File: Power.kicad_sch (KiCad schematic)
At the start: 38 parts, among them IC1 LM66200DRLR, J22 Conn_01x02, U10 LP2985-3.3, U9 AP63203WU

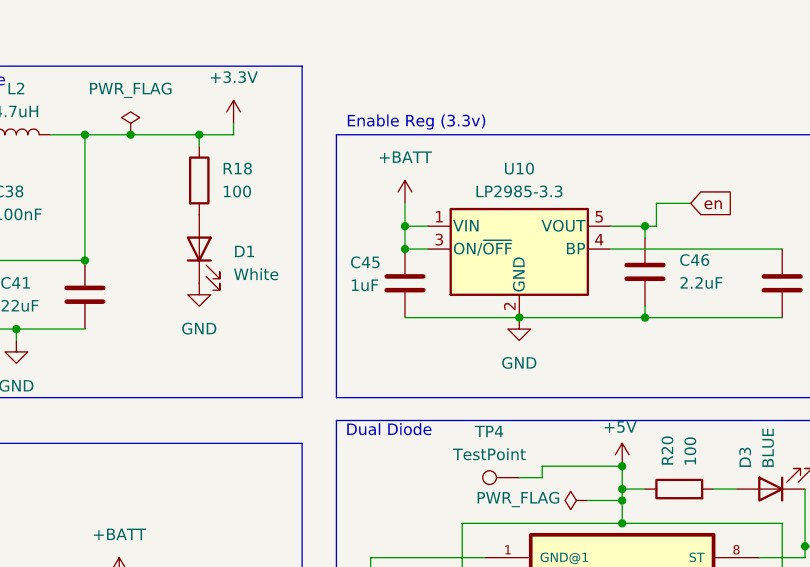
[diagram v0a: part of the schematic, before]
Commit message: v1.0 DONE6️⃣7️⃣🚀⚡️🔋
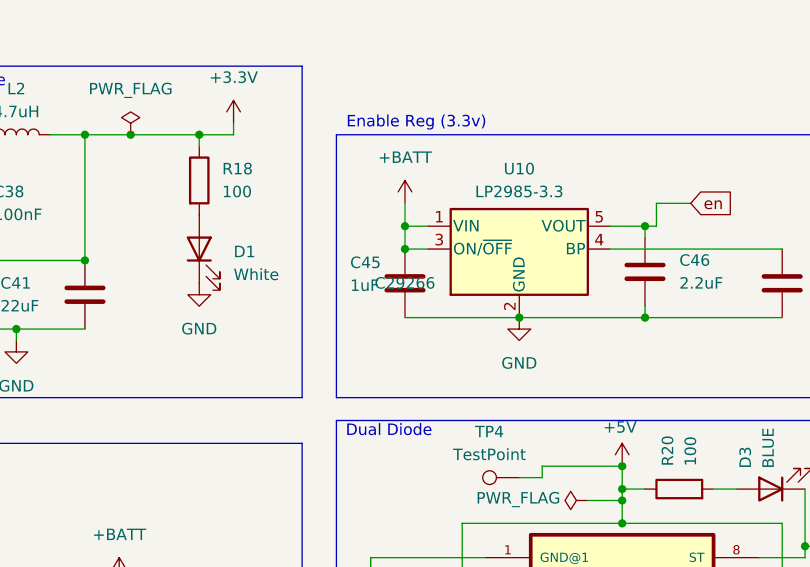
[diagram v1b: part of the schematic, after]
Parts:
- C45: JLC# (none) -> C29266
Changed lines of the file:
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@@
 			)
 		)
-		(property "JLC#" ""
+		(property "JLC#" "C29266"
 			(at 181.61 82.55 0)
 			(effects
